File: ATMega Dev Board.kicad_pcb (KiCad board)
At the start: 4 copper layers, 84 x 38.1 mm, 50 parts, among them J1 Conn_01x13, J2 Conn_01x09, J4 SPI header, J5 USB-C_31-M-12, Q1 S8050, Q2 2N7002, Q3 HL6042, Q4 HL6042, SW1 SW_SPST, SW2 SW_SPST, U1 ATmega32A-A, U2 CH340C, U3 USBLC6-2P6, X1 16MHz

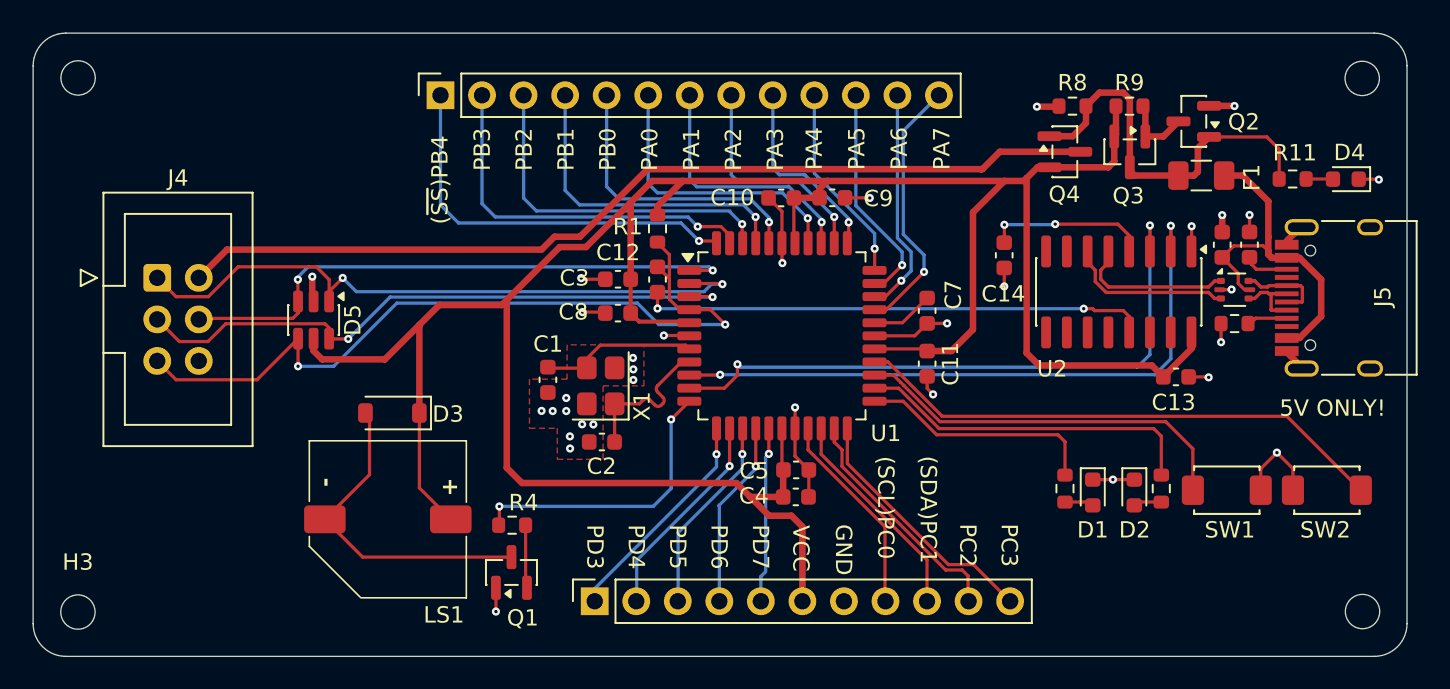
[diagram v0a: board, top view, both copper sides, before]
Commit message: updated constraints and traces
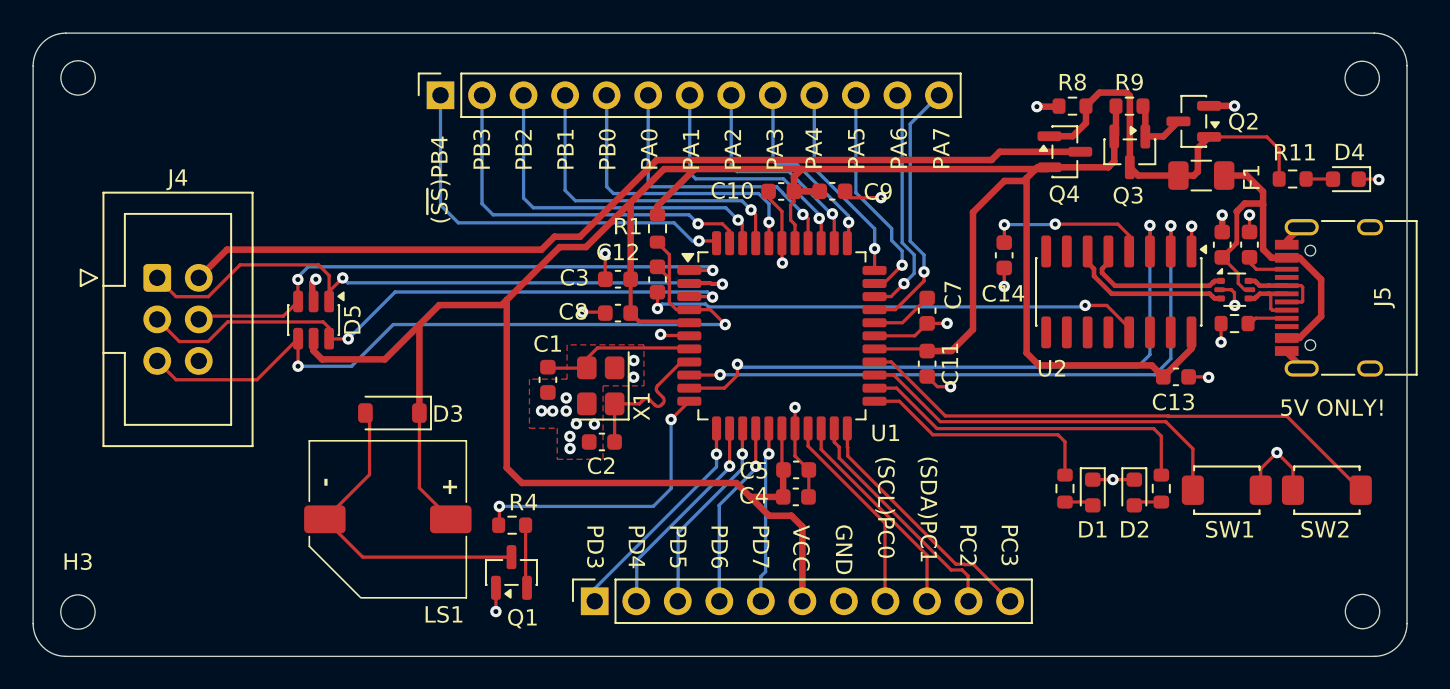
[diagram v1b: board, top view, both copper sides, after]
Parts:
- moved C10 0.40 mm to (83.6, 65.8)
- moved C9 0.40 mm to (86.7, 65.8)
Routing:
- net VCC: track 170.3 -> 175.3 mm
- net GND: track 48.0 -> 50.4 mm, vias 33 -> 32
- net VBUS: track 21.5 -> 23.4 mm
- net /RST: track 48.9 -> 48.0 mm
- net /UD_N: track 4.48 -> 5.32 mm
- net /PB0: track 17.8 -> 18.4 mm
